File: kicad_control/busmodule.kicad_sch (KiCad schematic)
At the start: 8 parts, among them U1 74LS163, U2 74LS163, U3 74LS163, U4 74LS163, U5 74LS244, U6 74LS244, U7 74LS374, U8 74LS374

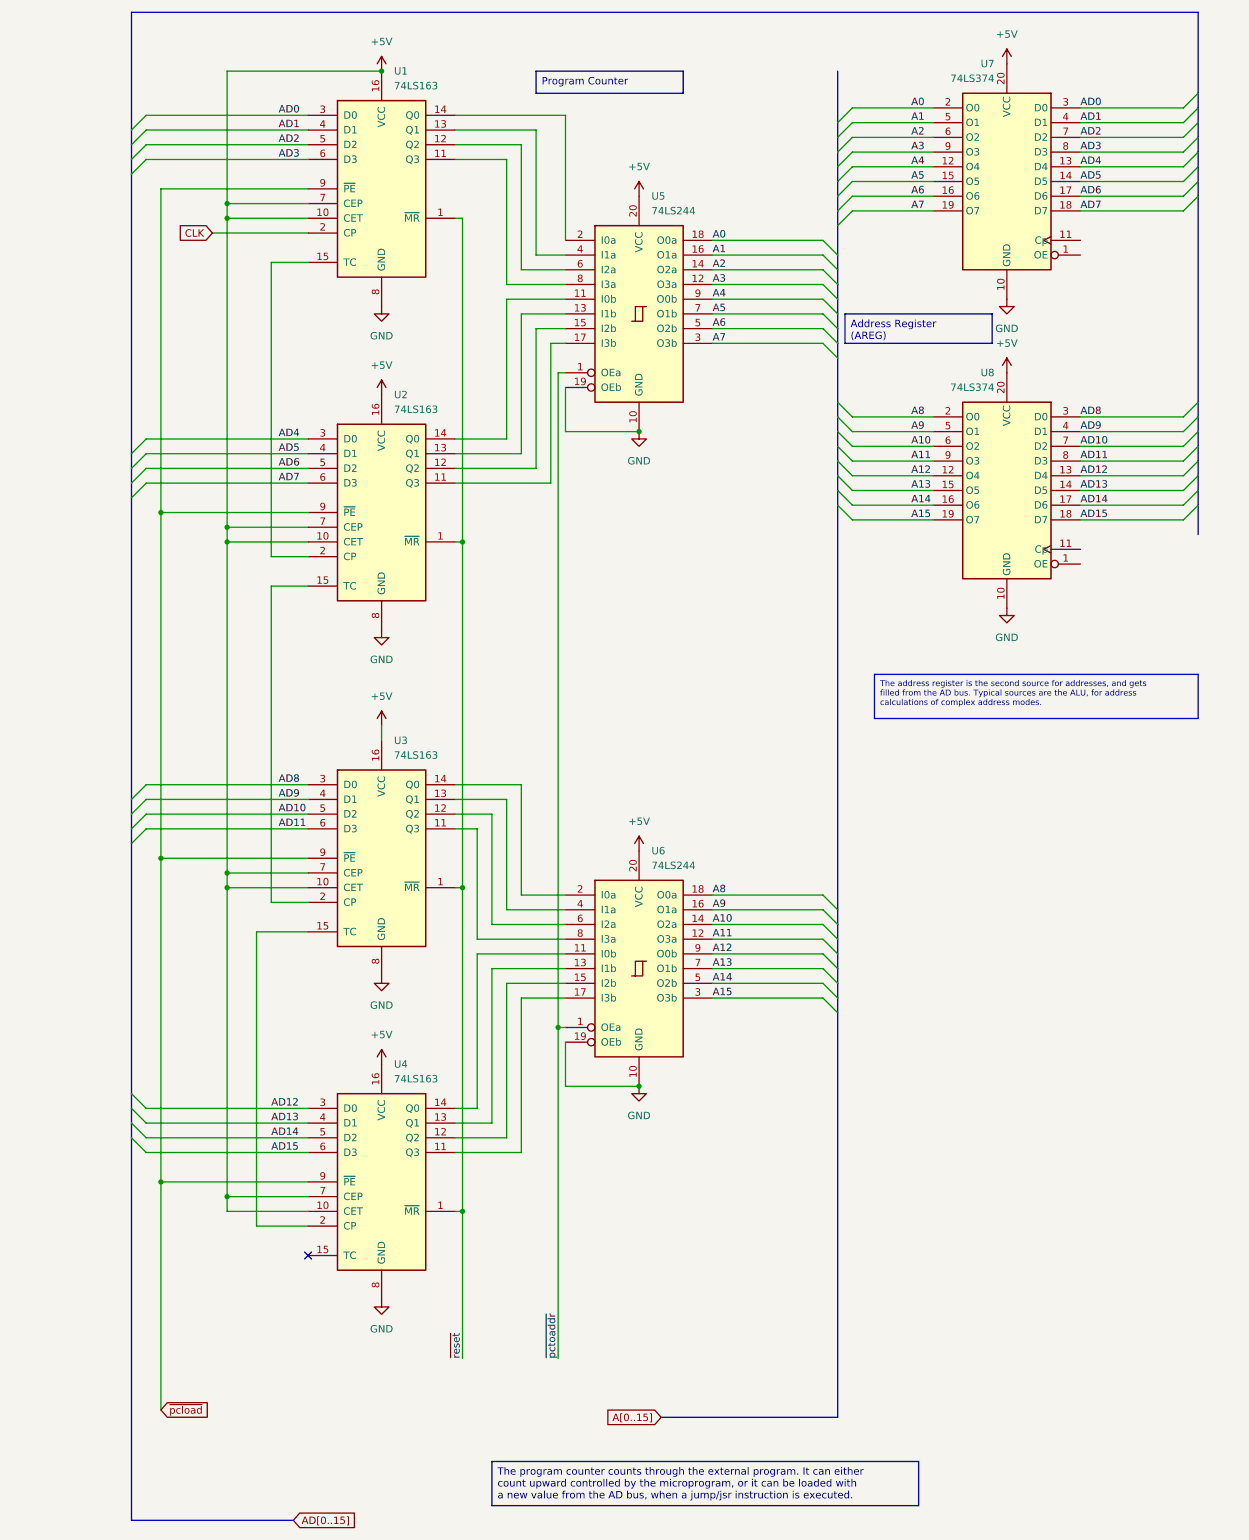
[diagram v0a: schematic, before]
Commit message: [control] work in progress
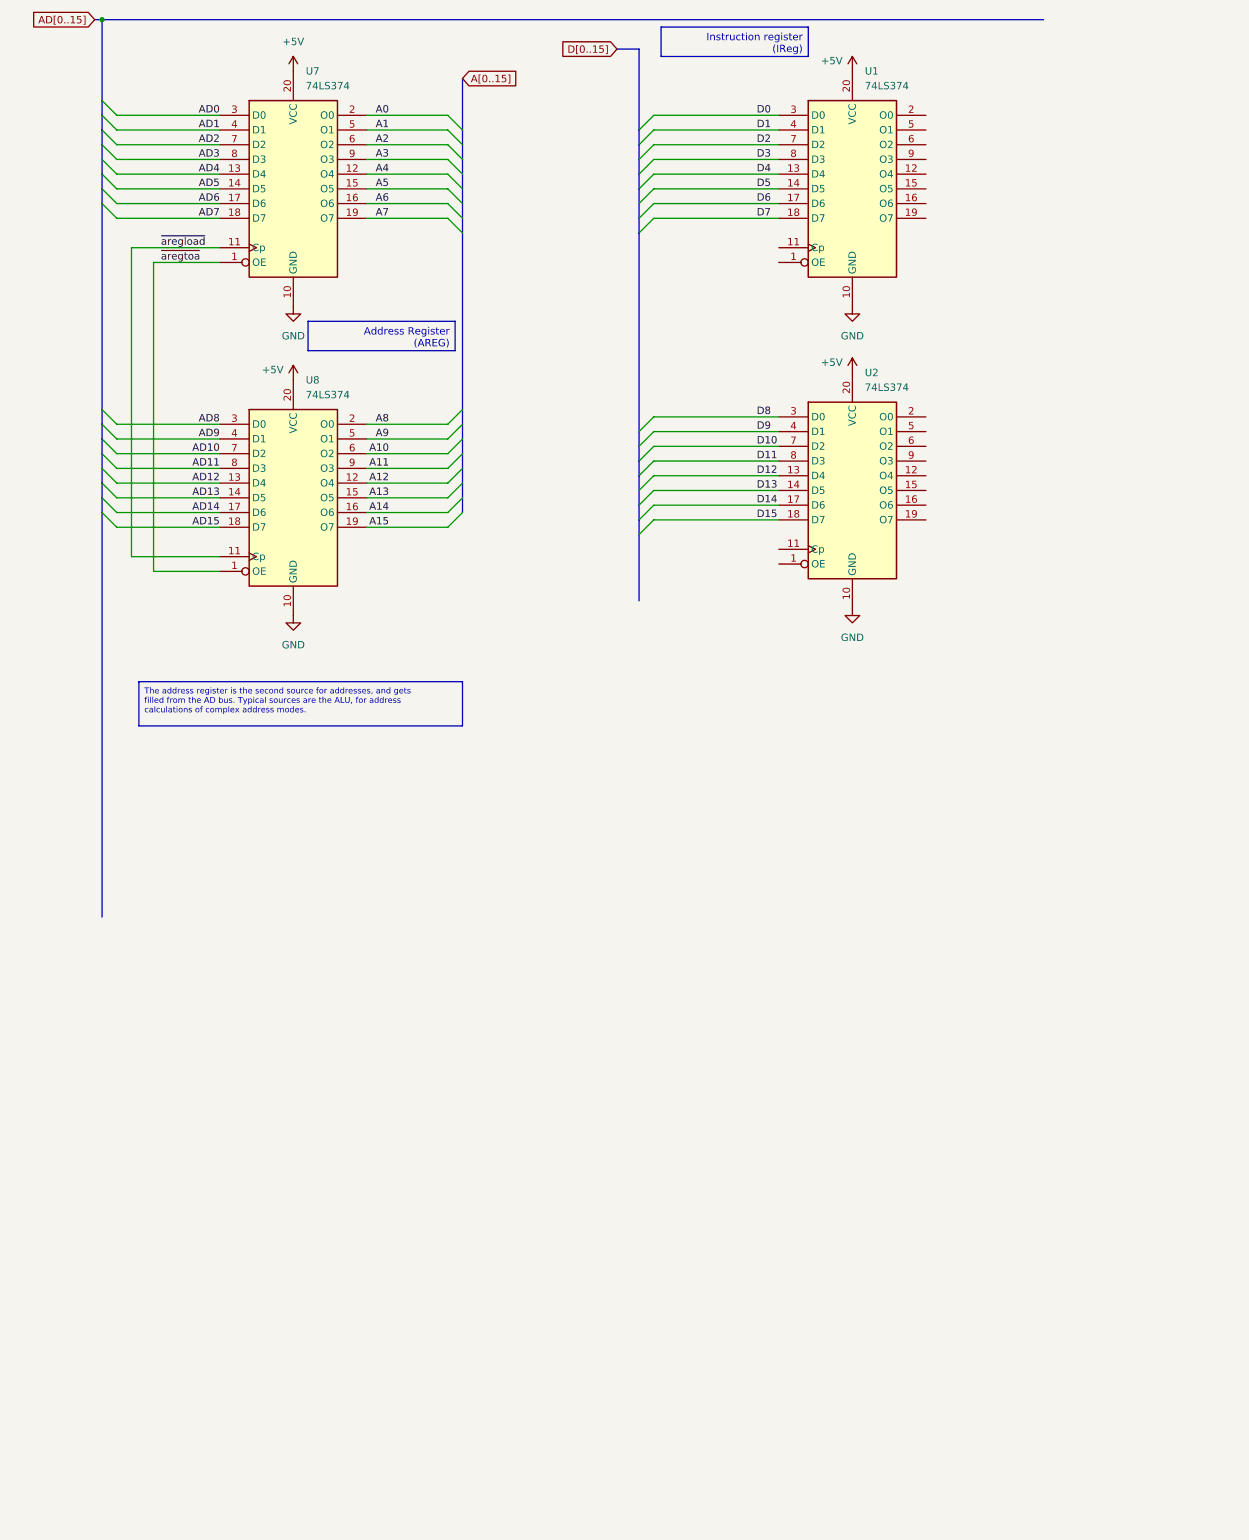
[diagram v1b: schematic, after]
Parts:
- removed U1, U2, U3, U4: 74LS163, symbol frits:74LS163
- removed U5, U6: 74LS244, symbol 74xx:74LS244
- added U1, U2: 74LS374, symbol 74xx:74LS374
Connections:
- net +5V: now also U1.20 (VCC), U2.20 (VCC)
- net GND: now also U1.10 (GND), U2.10 (GND)
- net ~{aregtoa}: now reaches U7.1 (OE)
- net ~{aregtoa}: now also U8.1 (OE)
- net ~{aregload}: now reaches U7.11 (Cp)
- net ~{aregload}: now also U8.11 (Cp)
- new net D0: U1.3 (D0)
- new net D1: U1.4 (D1)
- new net D10: U2.7 (D2)
- new net D11: U2.8 (D3)
- new net D12: U2.13 (D4)
- new net D13: U2.14 (D5)
- new net D14: U2.17 (D6)
- new net D15: U2.18 (D7)
- new net D2: U1.7 (D2)
- new net D3: U1.8 (D3)
- new net D4: U1.13 (D4)
- new net D5: U1.14 (D5)
- new net D6: U1.17 (D6)
- new net D7: U1.18 (D7)
- new net D8: U2.3 (D0)
- new net D9: U2.4 (D1)
- no-connect marks 1 -> 0
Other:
- moved on the sheet: U7, U8
